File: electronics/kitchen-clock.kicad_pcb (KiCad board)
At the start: 2 copper layers, 58.6 x 90.9 mm, 59 parts, among them IC1 CN3058E, IC2 HY2112, J1 USB_B_Micro, J2 INDICATORS, J3 PWR, J4 USB, J5 PWR, Q1 FS8205, Q2 2N7002, Q3 2N7002, SW1 SW_SPDT, U1 MT3608, U2 INA219AxD

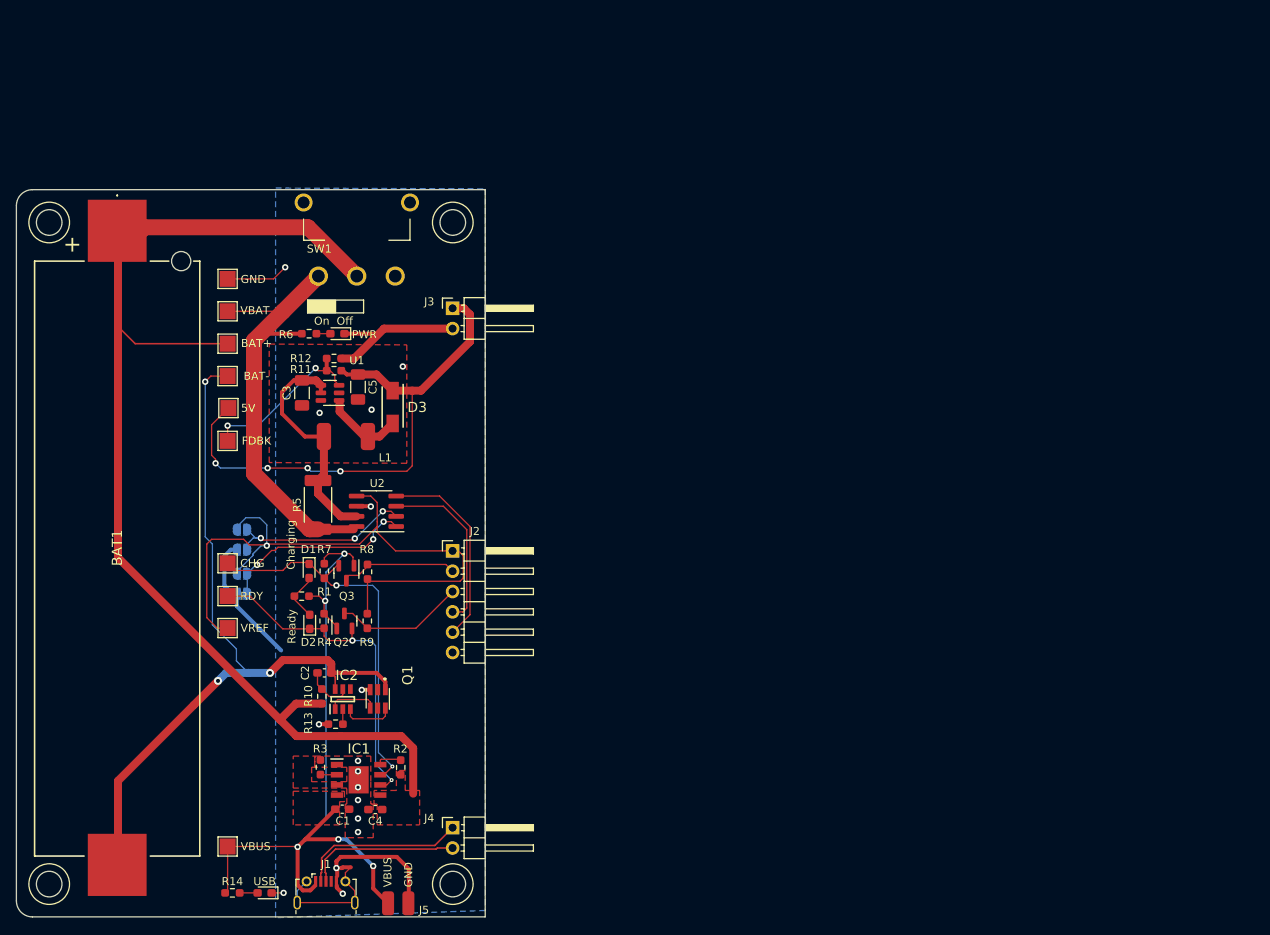
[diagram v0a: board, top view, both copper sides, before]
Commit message: First draft of schematic and PCB of controller board
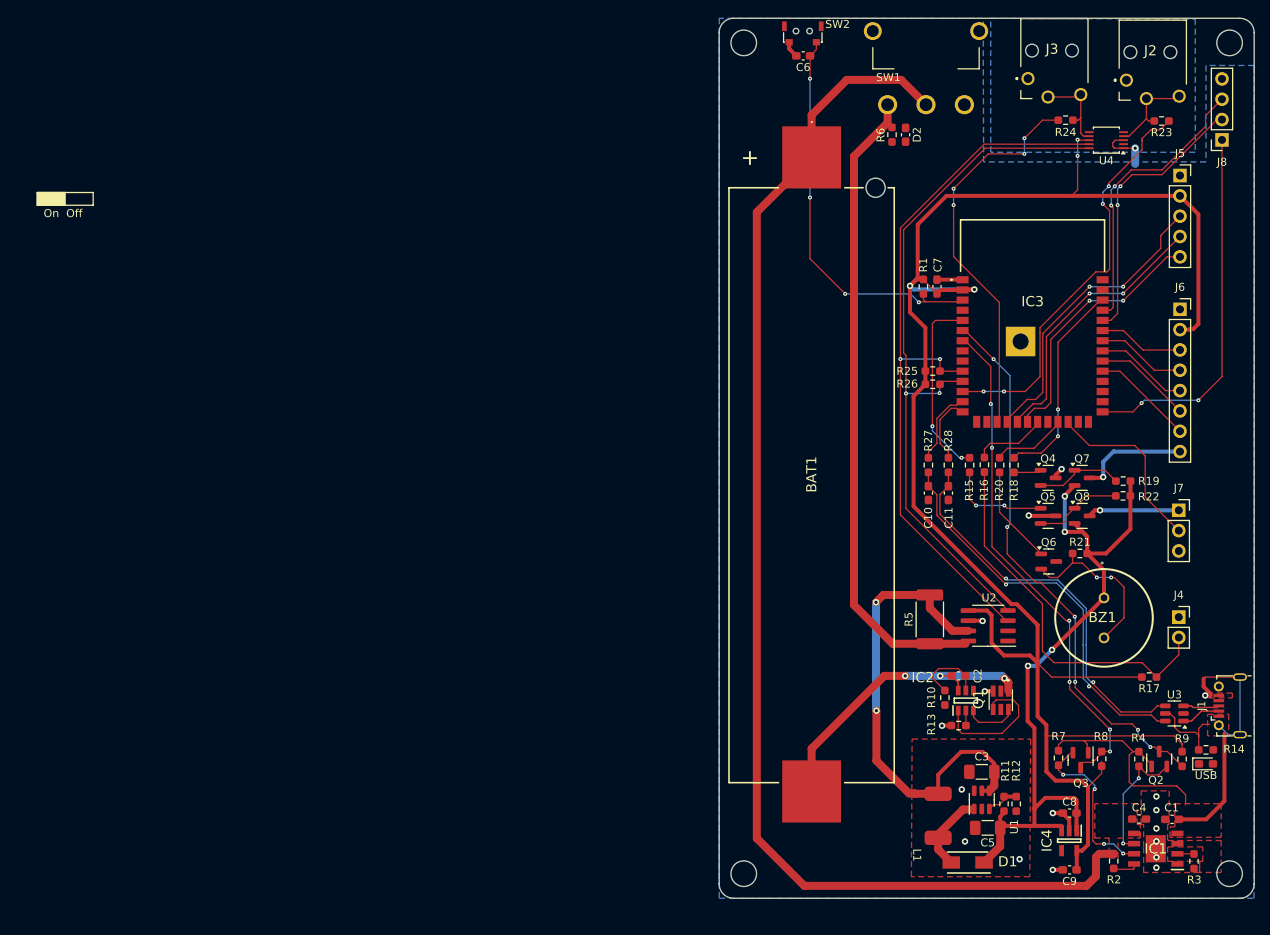
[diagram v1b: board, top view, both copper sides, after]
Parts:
- removed the D1 at (75.0, 107.0)
- removed the D2 at (75.1, 113.3)
- removed H1, H2, H3, H4: MountingHole, Chof747 Footprints:MountingHole_3.2mm_M3-smallBorder
- removed JP1: A1_H, Jumper:SolderJumper-2_P1.3mm_Open_RoundedPad1.0x1.5mm
- removed JP2: A1_L, Jumper:SolderJumper-2_P1.3mm_Open_RoundedPad1.0x1.5mm
- removed JP3: A0_H, Jumper:SolderJumper-2_P1.3mm_Open_RoundedPad1.0x1.5mm
- removed JP4: A0_L, Jumper:SolderJumper-2_P1.3mm_Open_RoundedPad1.0x1.5mm
- removed TP1: GND, TestPoint:TestPoint_Pad_2.0x2.0mm
- removed TP10: CHG, TestPoint:TestPoint_Pad_2.0x2.0mm
- removed TP2: VBAT, TestPoint:TestPoint_Pad_2.0x2.0mm
- removed TP3: BAT+, TestPoint:TestPoint_Pad_2.0x2.0mm
- removed TP4: BAT-, TestPoint:TestPoint_Pad_2.0x2.0mm
- removed TP5: 5V, TestPoint:TestPoint_Pad_2.0x2.0mm
- removed TP6: FDBK, TestPoint:TestPoint_Pad_2.0x2.0mm
- removed TP7: VBUS, TestPoint:TestPoint_Pad_2.0x2.0mm
- removed TP8: VREF, TestPoint:TestPoint_Pad_2.0x2.0mm
- removed TP9: RDY, TestPoint:TestPoint_Pad_2.0x2.0mm
- added BZ1: Buzzer, Chof747 Footprints:PS1240P02BT, F.Cu at (174.3, 112.8)
- added C10: 20p, Capacitor_SMD:C_0603_1608Metric_Pad1.08x0.95mm_HandSolder, F.Cu at (152.4, 97.2)
- added C11: 20p, Capacitor_SMD:C_0603_1608Metric_Pad1.08x0.95mm_HandSolder, F.Cu at (154.9, 97.2)
- added C6: 1uF, Capacitor_SMD:C_0603_1608Metric_Pad1.08x0.95mm_HandSolder, F.Cu at (136.8, 42.6)
- added C7: 10uF, Capacitor_SMD:C_0603_1608Metric_Pad1.08x0.95mm_HandSolder, F.Cu at (153.5, 71.4)
- added C8: 1uF, Capacitor_SMD:C_0603_1608Metric_Pad1.08x0.95mm_HandSolder, F.Cu at (170.1, 137.2)
- added C9: 1uF, Capacitor_SMD:C_0603_1608Metric_Pad1.08x0.95mm_HandSolder, F.Cu at (170.1, 144.3)
- added IC3: ESP32-S3-WROOM-1-N8R8, Chof747 Footprints:ESP32S3WROOM1N8R8, F.Cu at (165.4, 75.8)
- added IC4: ME6211C33M5G-N, Chof747 Footprints:SOT95P270X145-5N, F.Cu at (170.0, 140.7)
- added J6: CONN_DISPL, Connector_PinSocket_2.54mm:PinSocket_1x08_P2.54mm_Vertical, F.Cu at (183.8, 74.3)
- added J7: CONN_SERVO, Connector_PinSocket_2.54mm:PinSocket_1x03_P2.54mm_Vertical, F.Cu at (183.7, 99.4)
- added J8: CONN_PGR, Connector_PinSocket_2.54mm:PinSocket_1x04_P2.54mm_Vertical, F.Cu at (189.1, 53.1)
- added Q4: SS8050-G, Package_TO_SOT_SMD:SOT-23, F.Cu at (167.4, 95.3)
- added Q5: SS8050-G, Package_TO_SOT_SMD:SOT-23, F.Cu at (167.4, 100.1)
- added Q6: SS8050-G, Package_TO_SOT_SMD:SOT-23, F.Cu at (167.4, 105.8)
- added Q7: AO3401A, Package_TO_SOT_SMD:SOT-23, F.Cu at (171.6, 95.3)
- added Q8: AO3401A, Package_TO_SOT_SMD:SOT-23, F.Cu at (171.6, 100.1)
- added R15: 1k, Resistor_SMD:R_0603_1608Metric_Pad0.98x0.95mm_HandSolder, F.Cu at (157.6, 93.7)
- added R16: 1k, Resistor_SMD:R_0603_1608Metric_Pad0.98x0.95mm_HandSolder, F.Cu at (159.4, 93.7)
- added R17: 10k, Resistor_SMD:R_0603_1608Metric_Pad0.98x0.95mm_HandSolder, F.Cu at (180.0, 120.2)
- added R18: 1k, Resistor_SMD:R_0603_1608Metric_Pad0.98x0.95mm_HandSolder, F.Cu at (163.1, 93.7)
- added R19: 10k, Resistor_SMD:R_0603_1608Metric_Pad0.98x0.95mm_HandSolder, F.Cu at (176.8, 95.7)
- added R20: 1k, Resistor_SMD:R_0603_1608Metric_Pad0.98x0.95mm_HandSolder, F.Cu at (161.3, 93.7)
- added R21: 1k, Resistor_SMD:R_0603_1608Metric_Pad0.98x0.95mm_HandSolder, F.Cu at (171.3, 104.8)
- added R22: 10k, Resistor_SMD:R_0603_1608Metric_Pad0.98x0.95mm_HandSolder, F.Cu at (176.7, 97.6)
- added R23: 2k, Resistor_SMD:R_0603_1608Metric_Pad0.98x0.95mm_HandSolder, F.Cu at (181.6, 50.7)
- added R24: 2k, Resistor_SMD:R_0603_1608Metric_Pad0.98x0.95mm_HandSolder, F.Cu at (169.6, 50.6)
- added R25: 10k, Resistor_SMD:R_0603_1608Metric_Pad0.98x0.95mm_HandSolder, F.Cu at (152.9, 82.0)
- added R26: 10k, Resistor_SMD:R_0603_1608Metric_Pad0.98x0.95mm_HandSolder, F.Cu at (152.9, 83.6)
- added R27: 22, Resistor_SMD:R_0603_1608Metric_Pad0.98x0.95mm_HandSolder, F.Cu at (152.4, 93.7)
- added R28: 22, Resistor_SMD:R_0603_1608Metric_Pad0.98x0.95mm_HandSolder, F.Cu at (154.9, 93.7)
- added SW2: Reset, Chof747 Footprints:1TS003B-2500-3500A-CT (SMD Right Angle Tactile Switch), F.Cu at (136.7, 39.5)
- added U3: USBLC6-2SC6, Package_TO_SOT_SMD:SOT-23-6, F.Cu at (183.2, 124.8)
- added U4: ADS1115IDGS, Package_SO:TSSOP-10_3x3mm_P0.5mm, F.Cu at (174.7, 53.1)
- D2: renamed from D4; footprint LED_SMD:LED_0603_1608Metric_Pad1.05x0.95mm_HandSolder -> Capacitor_SMD:C_0603_1608Metric_Pad1.08x0.95mm_HandSolder
- J2: value INDICATORS -> Temp 1; footprint Connector_PinHeader_2.54mm:PinHeader_1x06_P2.54mm_Horizontal -> Chof747 Footprints:MJ2509N
- J3: value PWR -> Temp 2; footprint Connector_PinHeader_2.54mm:PinHeader_1x02_P2.54mm_Horizontal -> Chof747 Footprints:MJ2509N
- J4: value USB -> CONN_MOD; footprint Connector_PinHeader_2.54mm:PinHeader_1x02_P2.54mm_Horizontal -> Connector_PinSocket_2.54mm:PinSocket_1x02_P2.54mm_Vertical
- J5: value PWR -> CONN_ENC; footprint Chof747_Connectors:pad_1x2_1.5mmx3mm -> Connector_PinSocket_2.54mm:PinSocket_1x05_P2.54mm_Vertical
- R1: value 1k -> 10k
- moved J5 133.5 mm to (183.8, 57.5)
- moved R14 123.0 mm to (187.1, 129.3)
- moved D3 118.8 mm to (187.1, 131.1), turned to 0 degrees
- moved J1 115.3 mm to (190.1, 123.8), turned to 90 degrees
- moved R3 109.8 mm to (185.6, 143.2), turned to -90 degrees
- moved NT1 109.6 mm to (186.8, 120.9), turned to 90 degrees
- moved J2 107.8 mm to (182.2, 44.0), turned to 180 degrees
- moved C1 103.7 mm to (182.9, 138.0), turned to 180 degrees
- moved R4 103.3 mm to (178.7, 130.5)
- moved R9 103.3 mm to (184.1, 130.5)
- moved Q2 103.3 mm to (181.2, 130.5)
- moved R12 101.8 mm to (163.4, 136.1), turned to -90 degrees
- moved IC1 100.0 mm to (180.8, 141.7), turned to 180 degrees
- moved R11 99.7 mm to (161.9, 136.1), turned to 90 degrees
- moved C3 97.3 mm to (159.1, 132.1), turned to 180 degrees
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- renumbered D3 to D1, D5 to D3
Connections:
- net /boosted renamed /Battery Management/boosted
- net BAT+ renamed /Battery Management/BAT+
- net BAT- renamed /Battery Management/BAT-
- net CHG_IND renamed /Battery Management/CHG_IND
- net RDY_IND renamed /Battery Management/RDY_IND
- net VBAT renamed /Battery Management/VBAT
- net VBAT_M renamed /Battery Management/VBAT_M
- J2 pad 1: VREF -> GND
- J2 pad 2: Net-(J2-Pin_2) -> /Peripherals/TEMP0
- J2 pad 3: Net-(J2-Pin_3) -> /Peripherals/TEMP0
- J3 pad 1: +5V -> GND
- J3 pad 2: GND -> /Peripherals/TEMP1
- J4 pad 1: USB_N -> GND
- J4 pad 2: USB_P -> /Peripherals/MODE_BUTTON
- J5 pad 1: VBUS -> GND
- J5 pad 2: GND -> +3V3
- Q2 pad 3: Net-(J2-Pin_3) -> /Battery Management/READY
- Q3 pad 3: Net-(J2-Pin_2) -> /Battery Management/CHARGE
- R1 pad 1: VBUS -> +3V3
- R8 pad 1: VREF -> +3V3
- R8 pad 2: Net-(J2-Pin_2) -> /Battery Management/CHARGE
- R9 pad 1: VREF -> +3V3
- R9 pad 2: Net-(J2-Pin_3) -> /Battery Management/READY
- U2 pad 1: Net-(JP1-A) -> GND
- U2 pad 2: Net-(JP3-A) -> GND
- U2 pad 5: VREF -> +3V3
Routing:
- net +3V3: track 0.00 -> 224.2 mm, vias 0 -> 4
- net VREF: track 86.5 -> 0.00 mm, vias 1 -> 0
- net SDA: track 21.8 -> 92.0 mm, vias 0 -> 2
- net /Battery Management/READY: track 0.00 -> 69.1 mm, vias 0 -> 6
- net /Battery Management/CHARGE: track 0.00 -> 64.1 mm, vias 0 -> 6
- net SCL: track 24.9 -> 88.7 mm, vias 0 -> 2
- net /Battery Management/BAT-: track 98.4 -> 38.8 mm
- net /Microcontroller & Controls/ADC0_DRV_IO8: track 0.00 -> 51.3 mm, vias 0 -> 4
- net /Microcontroller & Controls/USBPROT_N: track 0.00 -> 50.5 mm, vias 0 -> 2
- net /Microcontroller & Controls/USBPROT_P: track 0.00 -> 49.7 mm, vias 0 -> 2
- net /Microcontroller & Controls/ADC1_DRV_IO9: track 0.00 -> 49.4 mm, vias 0 -> 4
- net /Peripherals/MODE_BUTTON: track 0.00 -> 47.1 mm
- net Net-(IC3-IO0): track 0.00 -> 46.3 mm, vias 0 -> 2
- net Net-(IC3-EN): track 6.15 -> 49.4 mm, vias 0 -> 4
- net GND: track 69.5 -> 27.7 mm, vias 16 -> 18
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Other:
- board size 58.6 x 90.9 mm -> 66.9 x 110 mm
- board text added: "KitchenClock v1.0 (2024)"
- board text removed: "Battery Power (LiFePo4) v1.0 (2024)"
- board text removed: "CHG IND"
- board text removed: "Charging"
- board text removed: "D+"
- board text removed: "D-"
- board text removed: "INA219 Adr."
- board text removed: "RDY IND"
- board text removed: "Ready"
- board text removed: "SCL(I2C)"
- board text removed: "SDA(I2C)"
- board text removed: "USB"
- board text removed: "VBUS"
- board text removed: "VREF"
